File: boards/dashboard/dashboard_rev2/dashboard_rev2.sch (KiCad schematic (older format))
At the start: 51 parts, among them IC1 ATMEGA16M1, J1 micromatch_male_10, J2 micromatch_male_14, J3 micromatch_female_RA_6, J4 NanoFit_2, P1 CONN_02X03, P2 CONN_02X03, U1 CAN_Transceiver, U2 TPS561201, U3 ATMEGA328P-AU, Y1 Crystal_SMD, Y2 Crystal_SMD

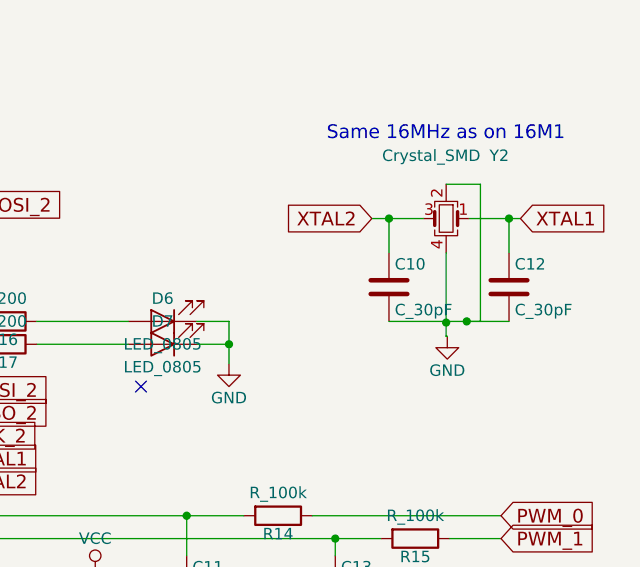
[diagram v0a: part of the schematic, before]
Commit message: Gerbers and PDFs
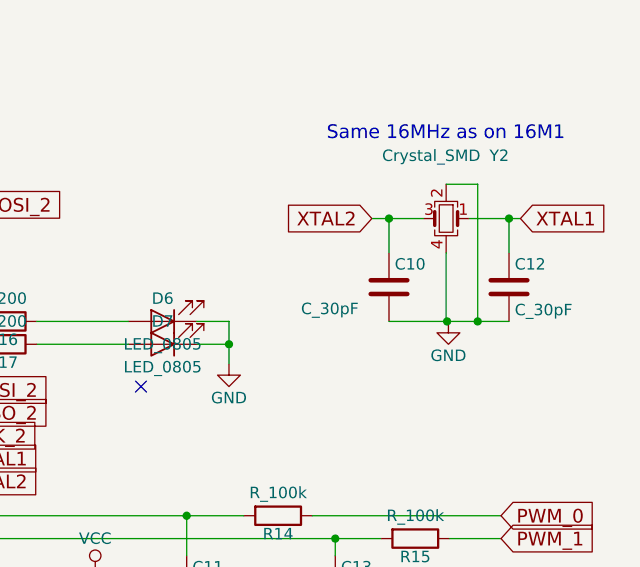
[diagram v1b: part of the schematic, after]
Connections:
- net GND: now also C10.2, C12.2, Y2.2
